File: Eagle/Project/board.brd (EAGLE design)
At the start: 44.1 x 47.7 mm, 18 parts, among them IC1 ATTINY402-SSF, X1 PAD-1.27X2.54, X2 PAD-1.27X2.54, X3 PAD-1.27X2.54

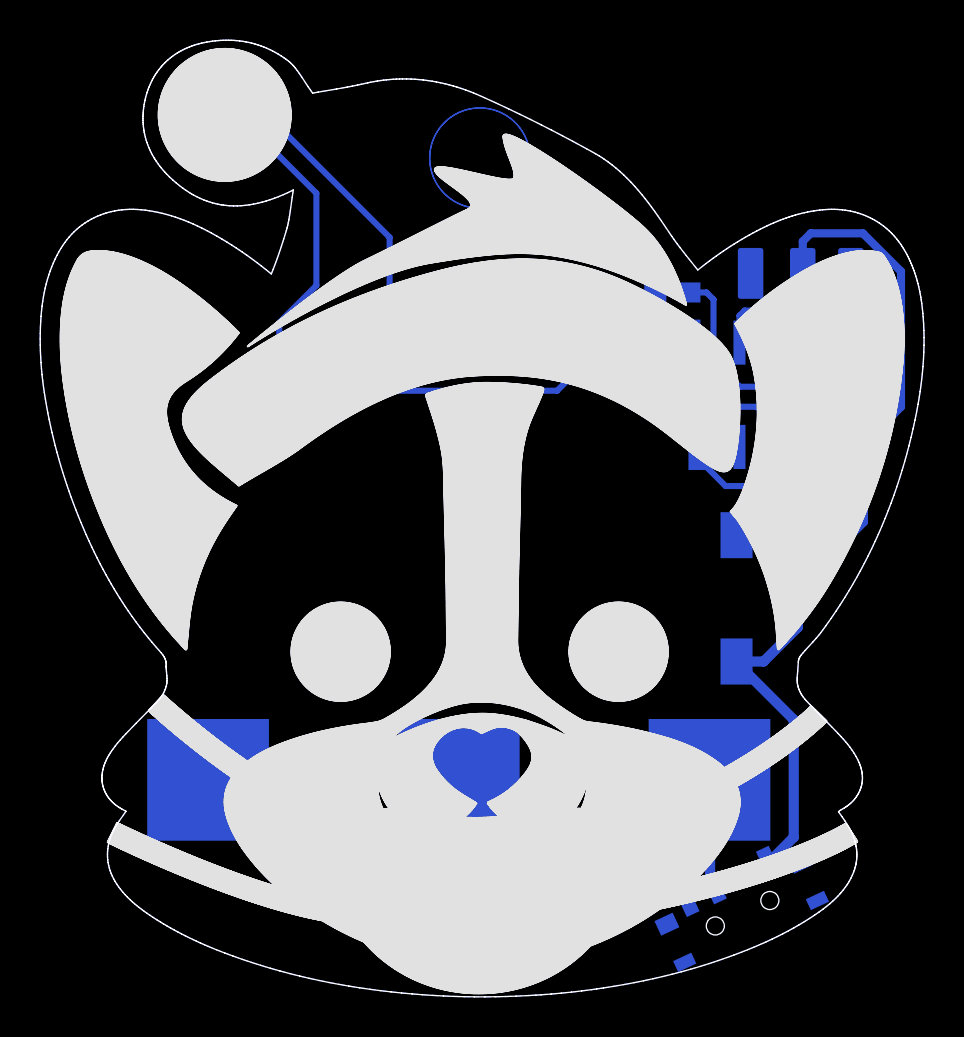
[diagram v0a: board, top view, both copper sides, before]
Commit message: Updated project
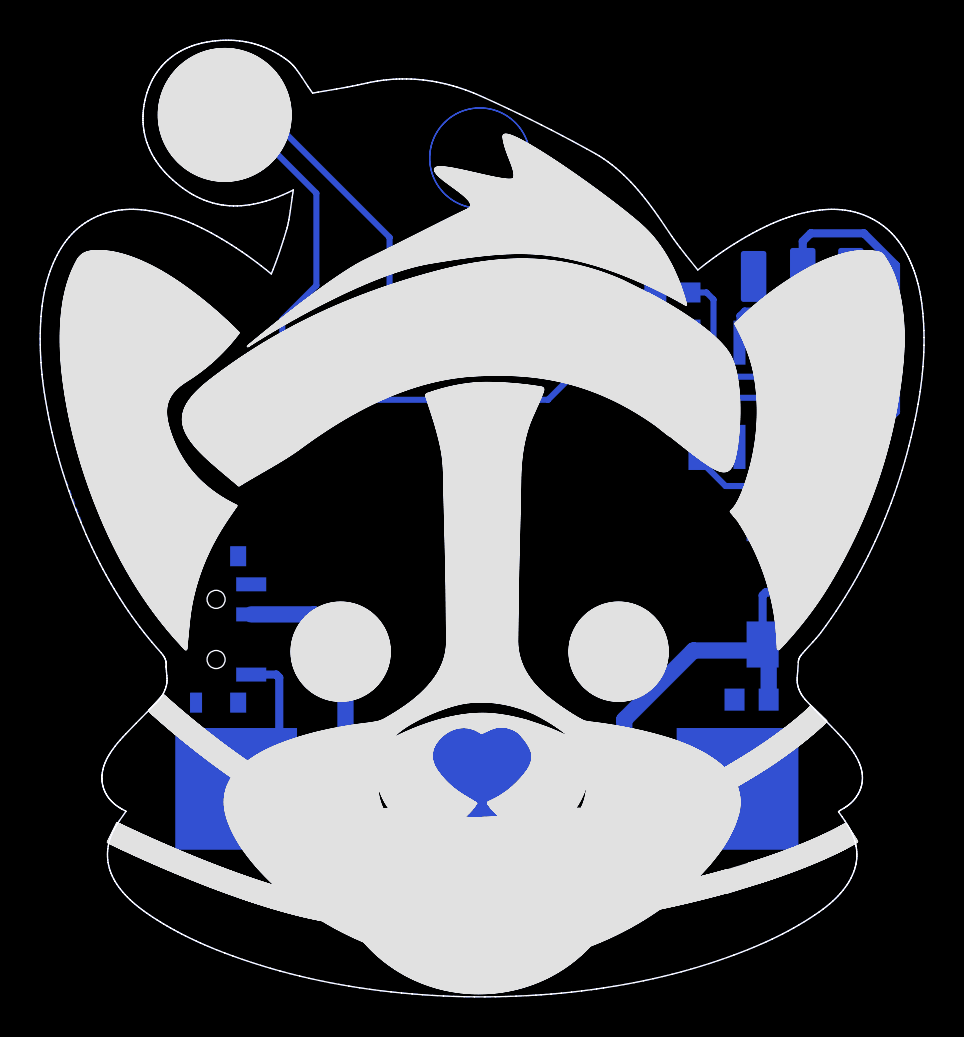
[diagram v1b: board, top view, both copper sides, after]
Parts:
- moved S2 29.8 mm to (12.3, 18.8), turned to 270 degrees
- moved R1 6.99 mm to (39.0, 15.3), turned to 180 degrees
- moved S1 1.55 mm to (39.6, 21.2)
- moved BT1 1.47 mm to (25.9, 10.8), turned to 180 degrees
- moved D6 0.71 mm to (14.3, 30.1)
- moved X3 0.21 mm to (39.1, 36.4)
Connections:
- removed net BAT+: BT1.1, S2.2
- new net N$6: BT1.1, S2.3
- net VCC: now also S2.2; no longer S2.3
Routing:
- net VCC: track 51.7 -> 87.1 mm
- net N$6: track 0.00 -> 8.37 mm
- net BAT+: track 5.74 -> 0.00 mm
- net N$2: track 7.98 -> 8.78 mm
